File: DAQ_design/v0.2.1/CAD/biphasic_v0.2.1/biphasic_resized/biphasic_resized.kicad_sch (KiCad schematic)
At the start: 26 parts, among them Q1 BC549, Q2 IRF9540N, Q3 IRF540N, Q4 BC549, Q5 IRF540N, Q6 IRF9540N

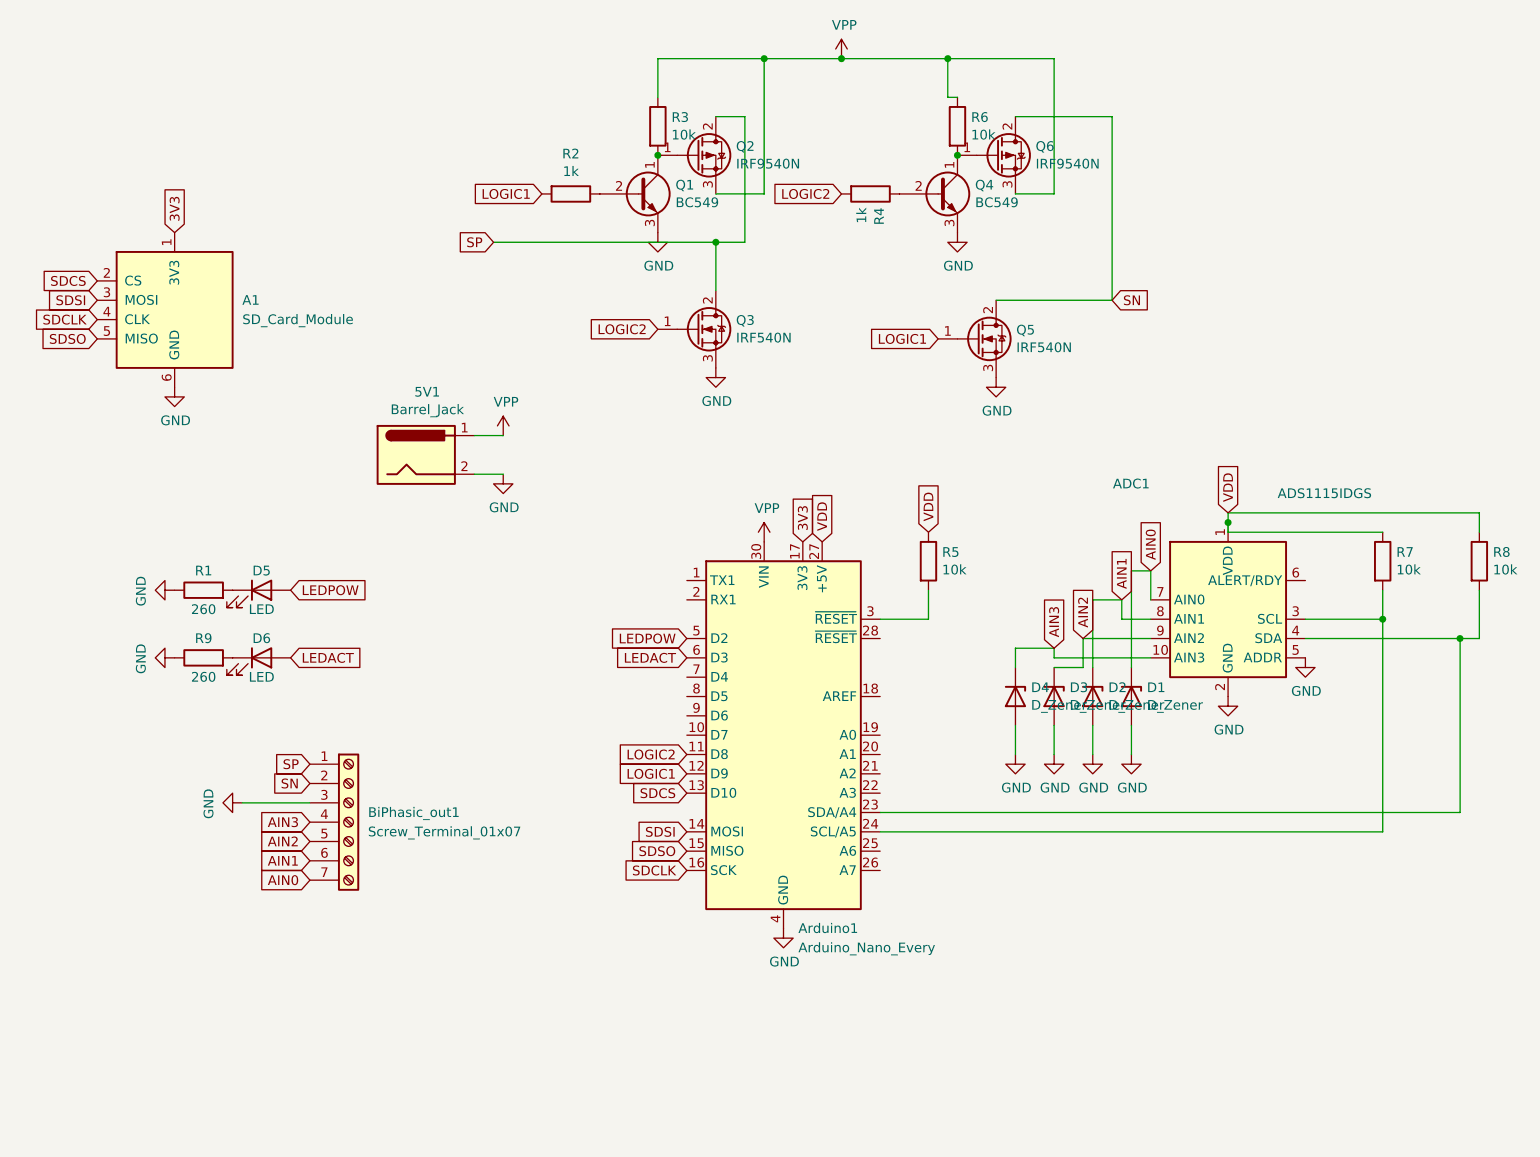
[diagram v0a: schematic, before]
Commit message: more tests
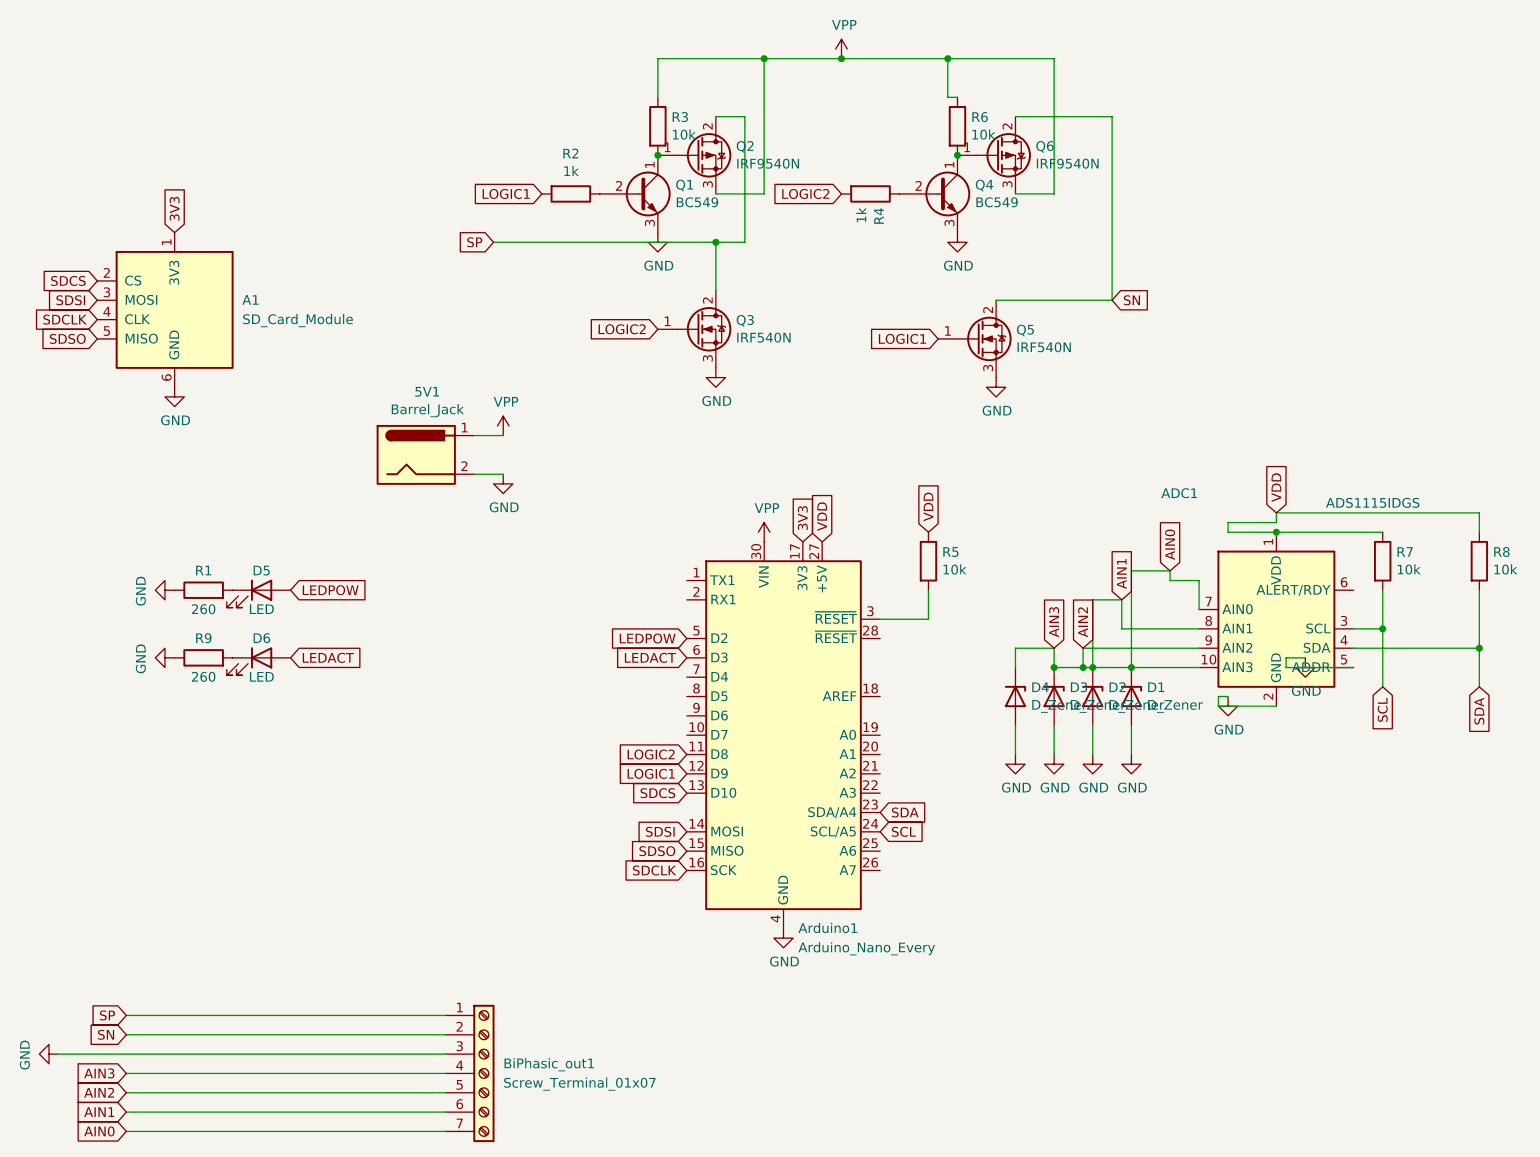
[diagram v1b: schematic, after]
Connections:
- net AIN1 is gone; now on net AIN0: ADC1.8 (AIN1), BiPhasic_out1.6 (Pin_6), D2.1 (K)
- net AIN2 is gone; now on net AIN0: ADC1.9 (AIN2), BiPhasic_out1.5 (Pin_5), D3.1 (K)
- net AIN3 is gone; now on net AIN0: ADC1.10 (AIN3), BiPhasic_out1.4 (Pin_4), D4.1 (K)
- net SCL: now reaches ADC1.3 (SCL), Arduino1.24 (SCL/A5), R7.2
- net SDA: now reaches ADC1.4 (SDA), Arduino1.23 (SDA/A4), R8.2
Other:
- moved on the sheet: ADC1, BiPhasic_out1
